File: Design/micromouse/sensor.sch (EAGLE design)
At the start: 9 parts

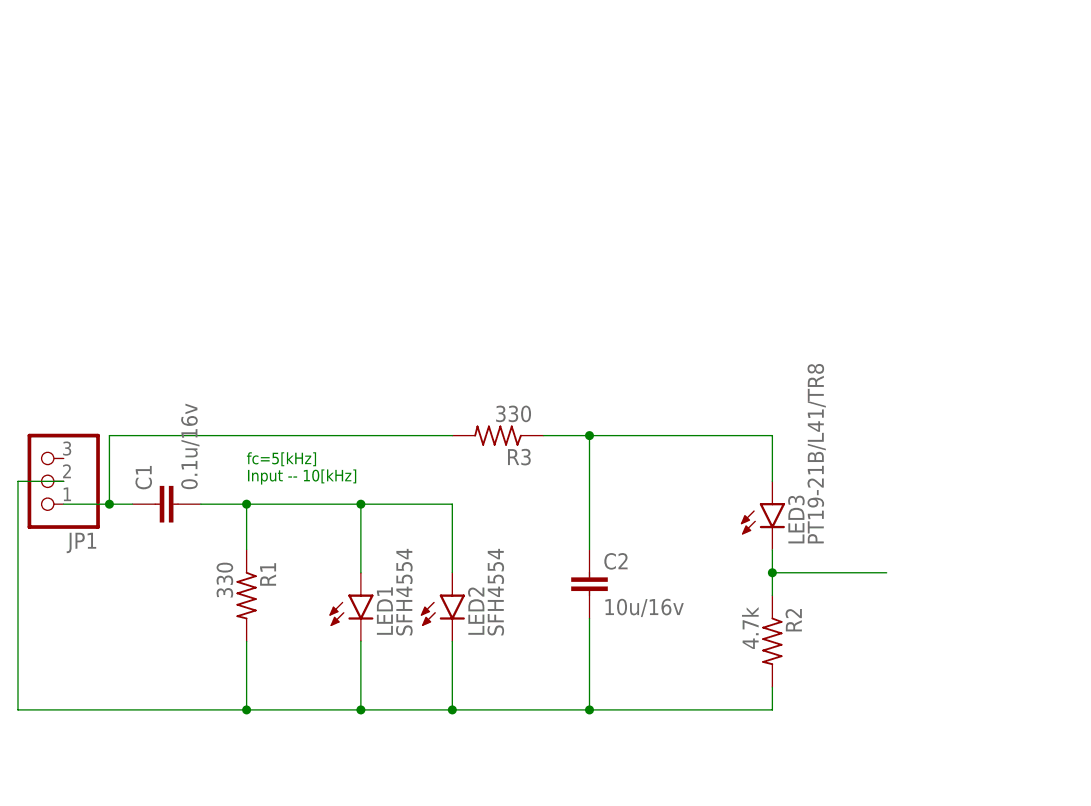
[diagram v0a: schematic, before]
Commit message: add firmware
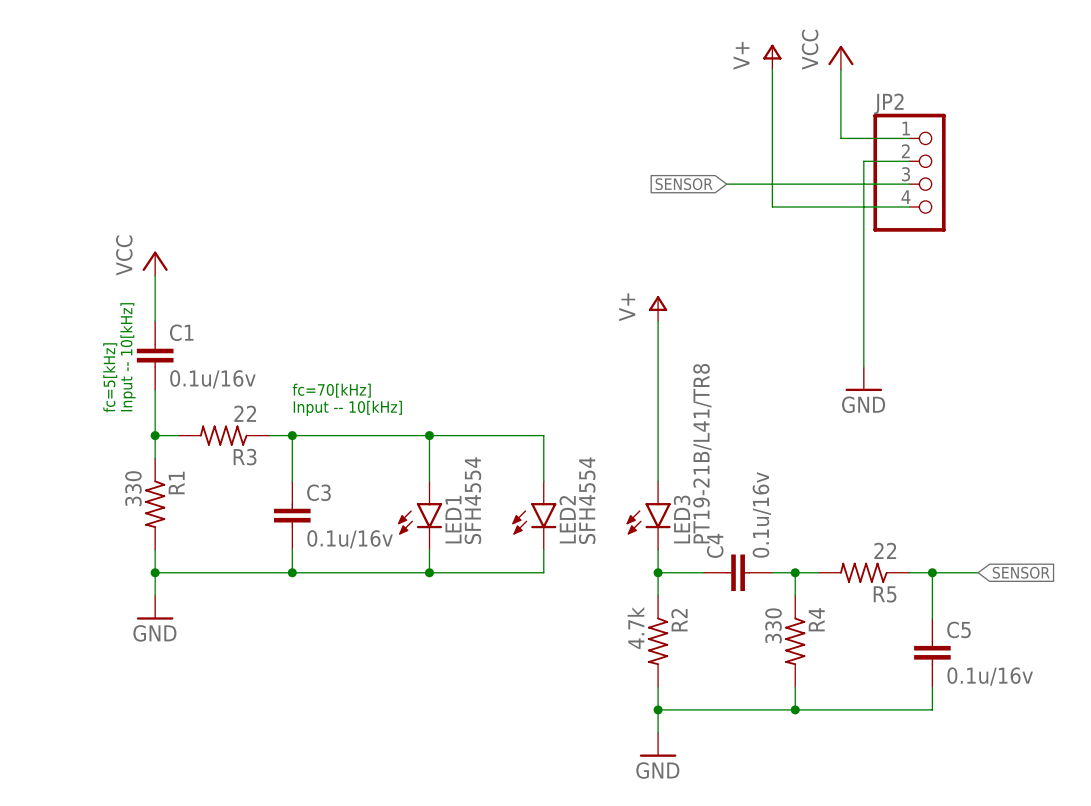
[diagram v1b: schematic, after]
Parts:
- removed C2: 10u/16v, rcl:C-EUC0603
- removed JP1: (no value), pinhead:PINHD-1X3/90
- added C3, C4, C5: 0.1u/16v, rcl:C-EUC0603
- added JP2: (no value), pinhead:PINHD-1X4/90
- added R4: 330, rcl:R-US_R0603
- added R5: 22, rcl:R-US_R0603
- R3: value 330 -> 22
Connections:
- removed net N$2: C2.2, JP1.2, LED1.C, LED2.C, R1.2, R2.2
- removed net N$3: C1.1, JP1.1, R3.2
- new net GND: C3.2, C5.2, JP2.2, LED1.C, LED2.C, R1.2, R2.2, R4.2
- new net N$10: C4.2, R4.1, R5.2
- new net SENSOR: C5.1, JP2.3, R5.1
- new net V+: JP2.4, LED3.A
- new net VCC: C1.1, JP2.1
- net N$1: now also C3.1, R3.1; no longer C1.2, R1.1
- net N$4: now also C4.1
- net N$5: now also C1.2, R1.1, R3.2; no longer C2.1, LED3.A, R3.1
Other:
- note added: "fc=70[kHz] Input -- 10[kHz]"
- moved on the sheet: C1, LED1, LED2, LED3, R1, R2, R3
